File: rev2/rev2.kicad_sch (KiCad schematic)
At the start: 74 parts, among them J101 Bluefruit LE, J102 Display, J103 JST-PH, SW101 Y, SW102 U, SW103 I, SW104 O, SW105 P, SW106 BSPC, SW107 H, SW108 J, SW109 K, SW110 L, SW111 ;, SW112 ENT, SW113 N, SW114 M, SW115 ,, SW116 ., SW117 /, SW118 RSHIFT, SW119 SPC, SW120 M1, SW121 M2, SW122 SUPER, U101 ATmega32U4, Y101 16 MHz

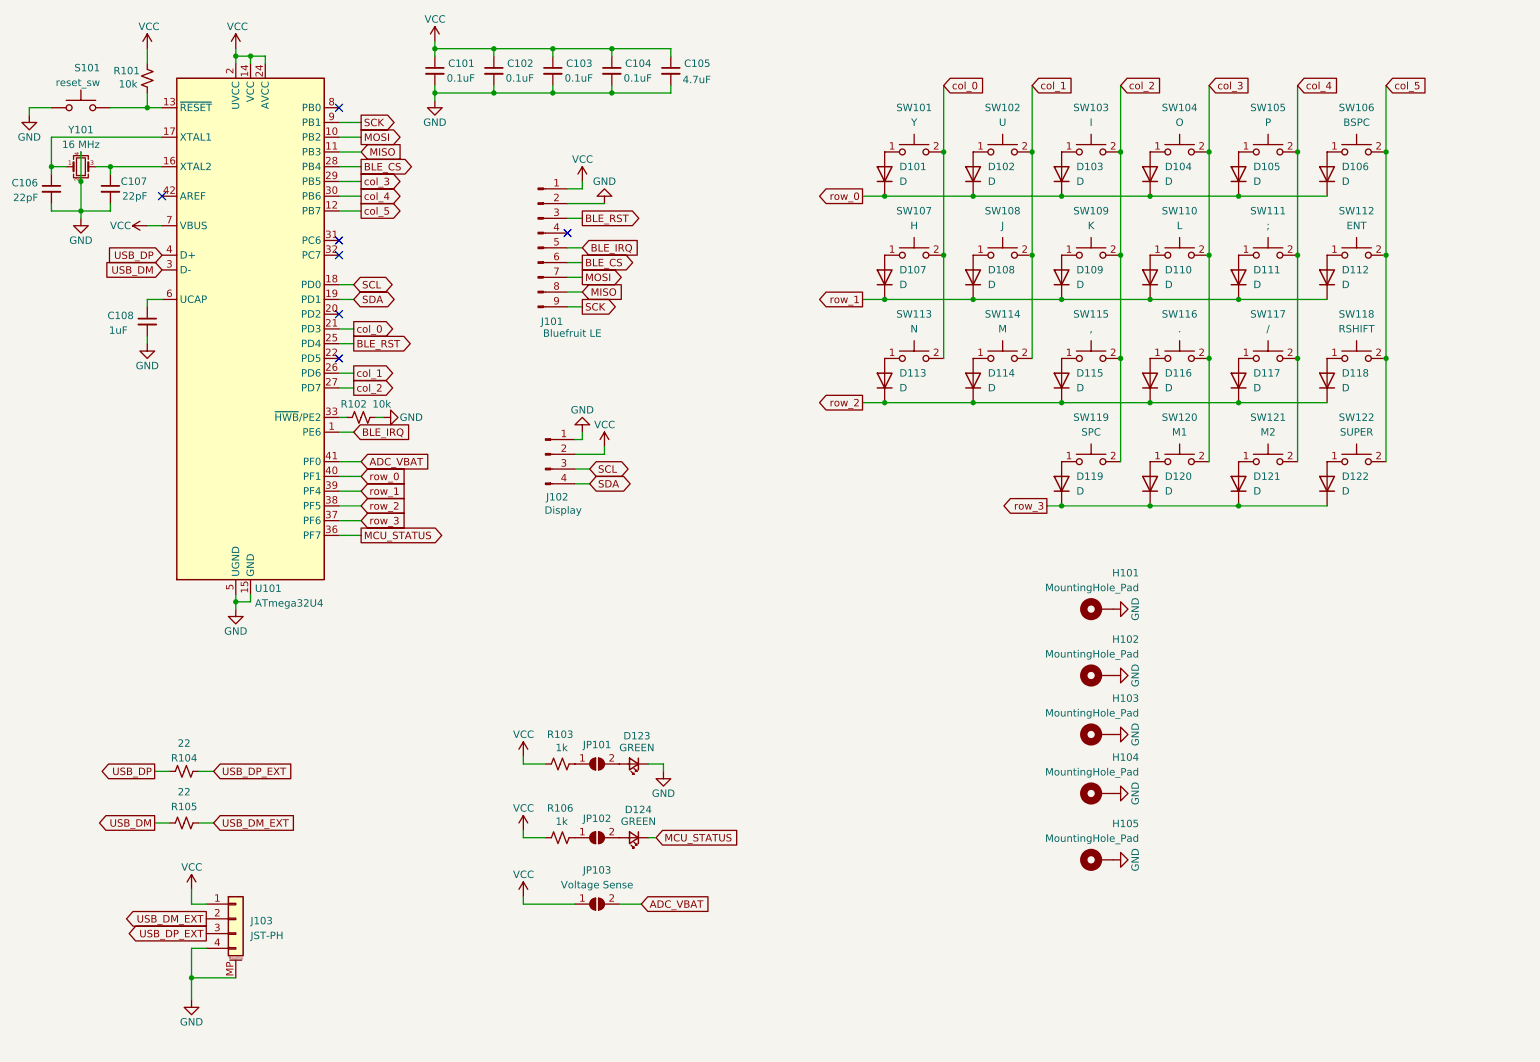
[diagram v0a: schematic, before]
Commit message: revision 1 and 2 added
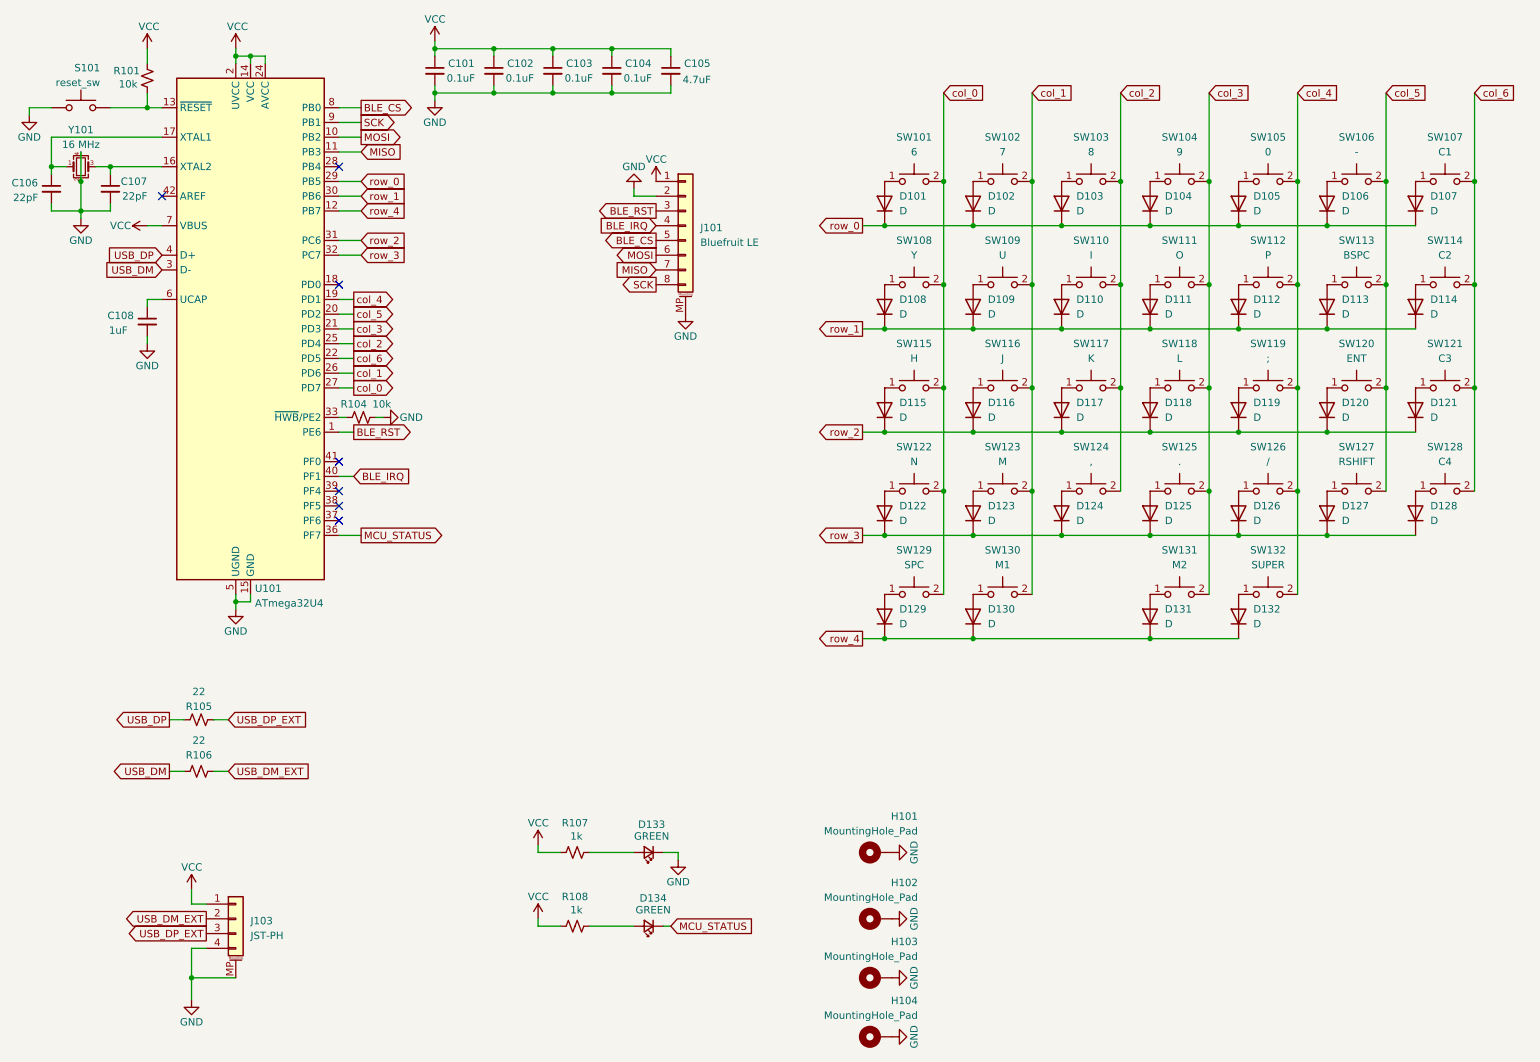
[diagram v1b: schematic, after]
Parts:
- removed H105: MountingHole_Pad, MountingHole:MountingHole_2.2mm_M2_Pad_TopBottom, symbol Mechanical:MountingHole_Pad
- removed J101: Bluefruit LE, Connector_PinHeader_2.54mm:PinHeader_1x09_P2.54mm_Vertical, symbol Connector:Conn_01x09_Pin
- removed J102: Display, Connector_PinHeader_2.54mm:PinHeader_1x04_P2.54mm_Vertical, symbol Connector:Conn_01x04_Pin
- removed JP101, JP102, JP103: Voltage Sense, Jumper:SolderJumper-2_P1.3mm_Open_Pad1.0x1.5mm, symbol Jumper:SolderJumper_2_Open
- added D101, D102, D103, D104, D105, D106, D107, D114, D121, D128: D, Diode_SMD:D_0603_1608Metric, symbol Device:D
- added J101: Bluefruit LE, Connector_JST:JST_SH_SM08B-SRSS-TB_1x08-1MP_P1.00mm_Horizontal, symbol Connector_Generic_MountingPin:Conn_01x08_MountingPin
- added SW101: 6, CherryMX_PCB:CherryMX_1.00u_PCB, symbol CherryMX:CherryMX
- added SW102: 7, CherryMX_PCB:CherryMX_1.00u_PCB, symbol CherryMX:CherryMX
- added SW103: 8, CherryMX_PCB:CherryMX_1.00u_PCB, symbol CherryMX:CherryMX
- added SW104: 9, CherryMX_PCB:CherryMX_1.00u_PCB, symbol CherryMX:CherryMX
- added SW105: 0, CherryMX_PCB:CherryMX_1.00u_PCB, symbol CherryMX:CherryMX
- added SW106: -, CherryMX_PCB:CherryMX_1.00u_PCB, symbol CherryMX:CherryMX
- added SW107: C1, CherryMX_PCB:CherryMX_1.00u_PCB, symbol CherryMX:CherryMX
- added SW114: C2, CherryMX_PCB:CherryMX_1.00u_PCB, symbol CherryMX:CherryMX
- added SW121: C3, CherryMX_PCB:CherryMX_1.00u_PCB, symbol CherryMX:CherryMX
- added SW128: C4, CherryMX_PCB:CherryMX_1.00u_PCB, symbol CherryMX:CherryMX
- J103: footprint Connector_JST:JST_PH_S4B-PH-SM4-TB_1x04-1MP_P2.00mm_Horizontal -> Connector_JST:JST_SH_SM04B-SRSS-TB_1x04-1MP_P1.00mm_Horizontal
- renumbered D101 to D108, D102 to D109, D103 to D110, D104 to D111, D105 to D112, D106 to D113, D107 to D115, D108 to D116, D109 to D117, D110 to D118, D111 to D119, D112 to D120, D113 to D122, D114 to D123, D115 to D124, D116 to D125, D117 to D126, D118 to D127, D119 to D129, D120 to D130, D121 to D131, D122 to D132, D123 to D133, D124 to D134, R102 to R104, R104 to R105, R105 to R106, R103 to R107, R106 to R108, SW101 to SW108, SW102 to SW109, SW103 to SW110, SW104 to SW111, SW105 to SW112, SW106 to SW113, SW107 to SW115, SW108 to SW116, SW109 to SW117, SW110 to SW118, SW111 to SW119, SW112 to SW120, SW113 to SW122, SW114 to SW123, SW115 to SW124, SW116 to SW125, SW117 to SW126, SW118 to SW127, SW119 to SW129, SW120 to SW130, SW121 to SW131, SW122 to SW132
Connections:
- net SDA is gone; now on net col_4: U101.19 (PD1)
- net BLE_CS: now also U101.8 (PB0), J101.5 (Pin_5); no longer U101.28 (PB4)
- net BLE_IRQ: now also U101.40 (PF1), J101.4 (Pin_4); no longer U101.1 (PE6)
- net BLE_RST: now also U101.1 (PE6), J101.3 (Pin_3); no longer U101.25 (PD4)
- net GND: now also J101.2 (Pin_2), J101.MP (MountPin)
- net MISO: now also J101.7 (Pin_7)
- net MOSI: now also J101.6 (Pin_6)
- net SCK: now also J101.8 (Pin_8)
- net VCC: now also J101.1 (Pin_1)
- net col_0: now also SW129.2, U101.27 (PD7), SW101.2; no longer U101.21 (PD3)
- net col_1: now also SW130.2, SW102.2
- net col_2: now also U101.25 (PD4), SW103.2; no longer SW129.2, U101.27 (PD7)
- net col_3: now also SW131.2, U101.21 (PD3), SW104.2; no longer SW130.2, U101.29 (PB5)
- net col_4: now also SW132.2, SW105.2; no longer SW131.2, U101.30 (PB6)
- net col_5: now also U101.20 (PD2), SW106.2; no longer SW132.2, U101.12 (PB7)
- net row_0: now also U101.29 (PB5), D101.1 (K), D102.1 (K), D103.1 (K), D104.1 (K), D105.1 (K), D106.1 (K), D107.1 (K); no longer D108.1 (K), D109.1 (K), D110.1 (K), D111.1 (K), D112.1 (K), D113.1 (K), U101.40 (PF1)
- net row_1: now also D108.1 (K), D109.1 (K), D110.1 (K), D111.1 (K), D112.1 (K), D113.1 (K), U101.30 (PB6), D114.1 (K); no longer D115.1 (K), D116.1 (K), D117.1 (K), D118.1 (K), D119.1 (K), D120.1 (K), U101.39 (PF4)
- net row_2: now also D115.1 (K), D116.1 (K), D117.1 (K), D118.1 (K), D119.1 (K), D120.1 (K), U101.31 (PC6), D121.1 (K); no longer D122.1 (K), D123.1 (K), D124.1 (K), D125.1 (K), D126.1 (K), D127.1 (K), U101.38 (PF5)
- net row_3: now also D122.1 (K), D123.1 (K), D124.1 (K), D125.1 (K), D126.1 (K), D127.1 (K), U101.32 (PC7), D128.1 (K); no longer D129.1 (K), D130.1 (K), D131.1 (K), D132.1 (K), U101.37 (PF6)
- net at R107.2: now also D133.2 (A)
- net col_6: now reaches U101.22 (PD5)
- net col_6: now also SW107.2, SW114.2, SW121.2, SW128.2
- net at R108.2: now also D134.2 (A)
- net ADC_VBAT: no longer names the net of U101.41 (PF0)
- net SCL: no longer names the net of U101.18 (PD0)
- new net: D103.2 (A), SW103.1
- new net: D101.2 (A), SW101.1
- new net: D114.2 (A), SW114.1
- new net: D102.2 (A), SW102.1
- new net: D105.2 (A), SW105.1
- new net: D107.2 (A), SW107.1
- new net: D121.2 (A), SW121.1
- new net: D106.2 (A), SW106.1
- new net: D128.2 (A), SW128.1
- new net: D104.2 (A), SW104.1
- new net row_4: D129.1 (K), D130.1 (K), D131.1 (K), D132.1 (K), U101.12 (PB7)
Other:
- moved on the sheet: D108, D109, D110, D111, D112, D113, D115, D116, D117, D118, D119, D120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
